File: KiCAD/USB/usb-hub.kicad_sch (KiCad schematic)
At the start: 20 parts, among them J1 Conn_01x10_Pin, J2 Conn_01x10_Pin, J3 Conn_01x04_Socket, U1 CY7C65634-28LTXC, Y1 12mHz 20pF

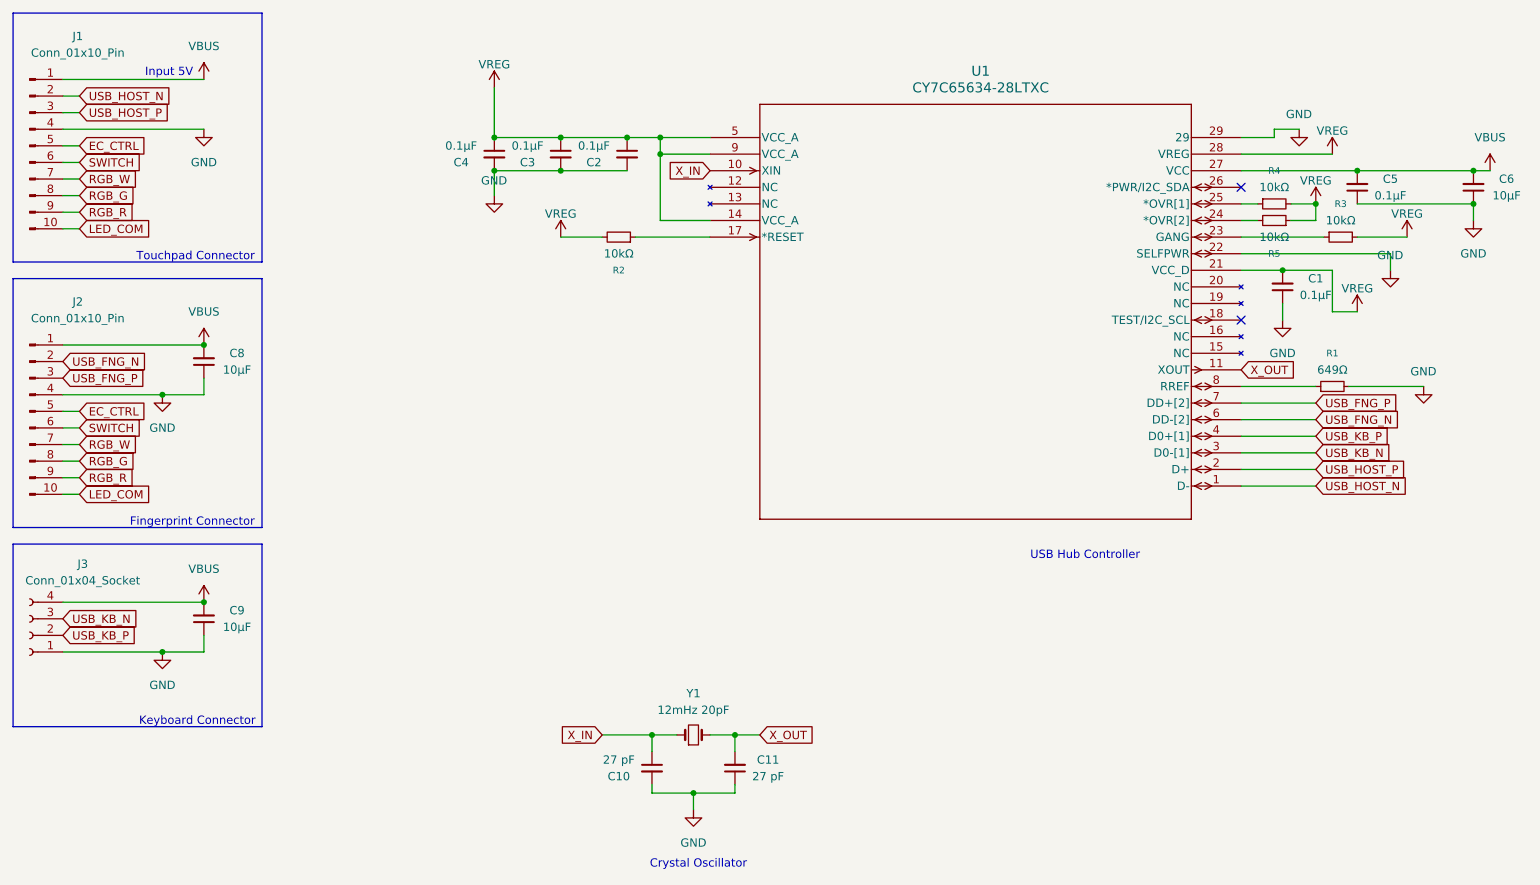
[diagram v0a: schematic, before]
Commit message: change symbol
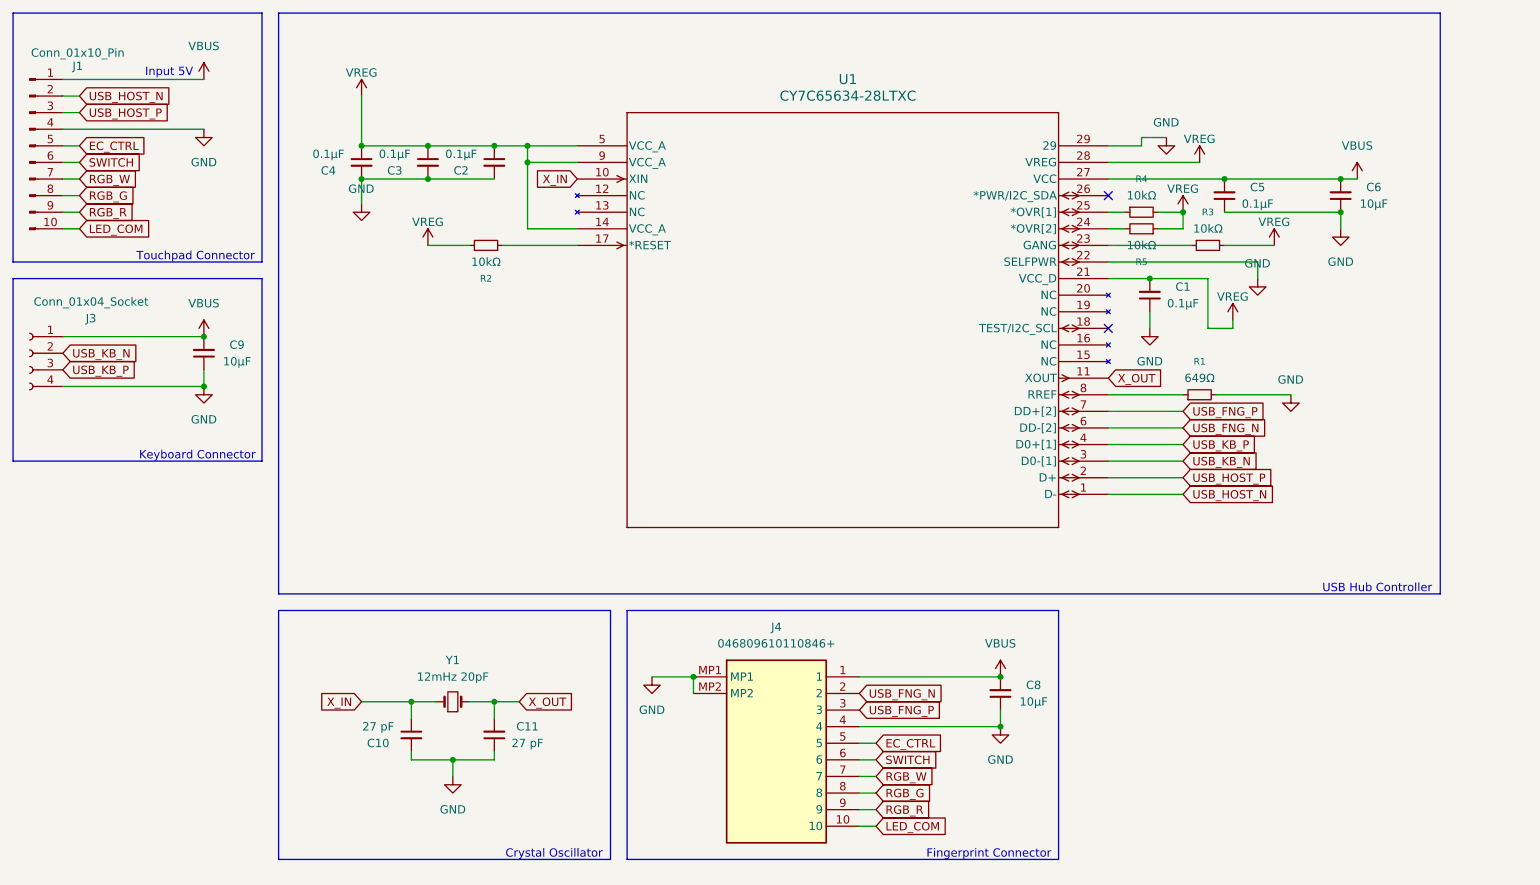
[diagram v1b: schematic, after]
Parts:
- removed J2: Conn_01x10_Pin, symbol Connector:Conn_01x10_Pin
- added J4: 046809610110846+, 046809610110846, symbol 046809610110846+:046809610110846+
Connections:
- net EC_CTRL: now also J4.5
- net GND: now also J3.4 (Pin_4), J4.4, J4.MP1, J4.MP2; no longer J3.1 (Pin_1)
- net LED_COM: now also J4.10
- net RGB_G: now also J4.8
- net RGB_R: now also J4.9
- net RGB_W: now also J4.7
- net SWITCH: now also J4.6
- net USB_FNG_N: now also J4.2
- net USB_FNG_P: now also J4.3
- net USB_KB_N: now also J3.2 (Pin_2); no longer J3.3 (Pin_3)
- net USB_KB_P: now also J3.3 (Pin_3); no longer J3.2 (Pin_2)
- net VBUS: now also J3.1 (Pin_1), J4.1; no longer J3.4 (Pin_4)
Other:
- moved on the sheet: C1, C10, C11, C2, C3, C4, C5, C6, C8, C9, J3, R1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
